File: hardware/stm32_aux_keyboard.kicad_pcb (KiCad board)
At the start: 2 copper layers, 95 x 95 mm, 188 parts, among them J1 I2C_HEADER,2.54, J2 WS2812_HEADER, J3 BUZZER_HEADER, J4 ROT_ENC_HEADER, J5 SWD_SWD, J6 SWD_SWD, J7 ROT_ENC_HEADER, J8 I2C_HEADER,2.54, Q1 SS9013_J3, SW1 USR_BTN_1, SW10 KEY22, SW11 KEY23, SW12 KEY31, SW13 KEY32, SW14 KEY33, SW18 ROT1, SW19 SW_RESET,2_leg,SMD, SW2 USR_BTN_2, SW3 USR_BTN_3, SW5 ROT2, SW6 KEY11, SW7 KEY12, SW8 KEY13, SW9 KEY21, U1 SSD1306-OLED-I2C, U10 STM32F103C8T6, U2 AMS1117-3.3, U3 74AHCT1G125, U4 USB, U5 USBLC6-2SC6_SOT23-6, U6 STM32F103C8T6_rect, U7 SWD, U8 AMS1117-3.3, U9 USBLC6-2SC6_SOT23-6, Y1 O_8M, Y2 O8M, Y3 O32.768K

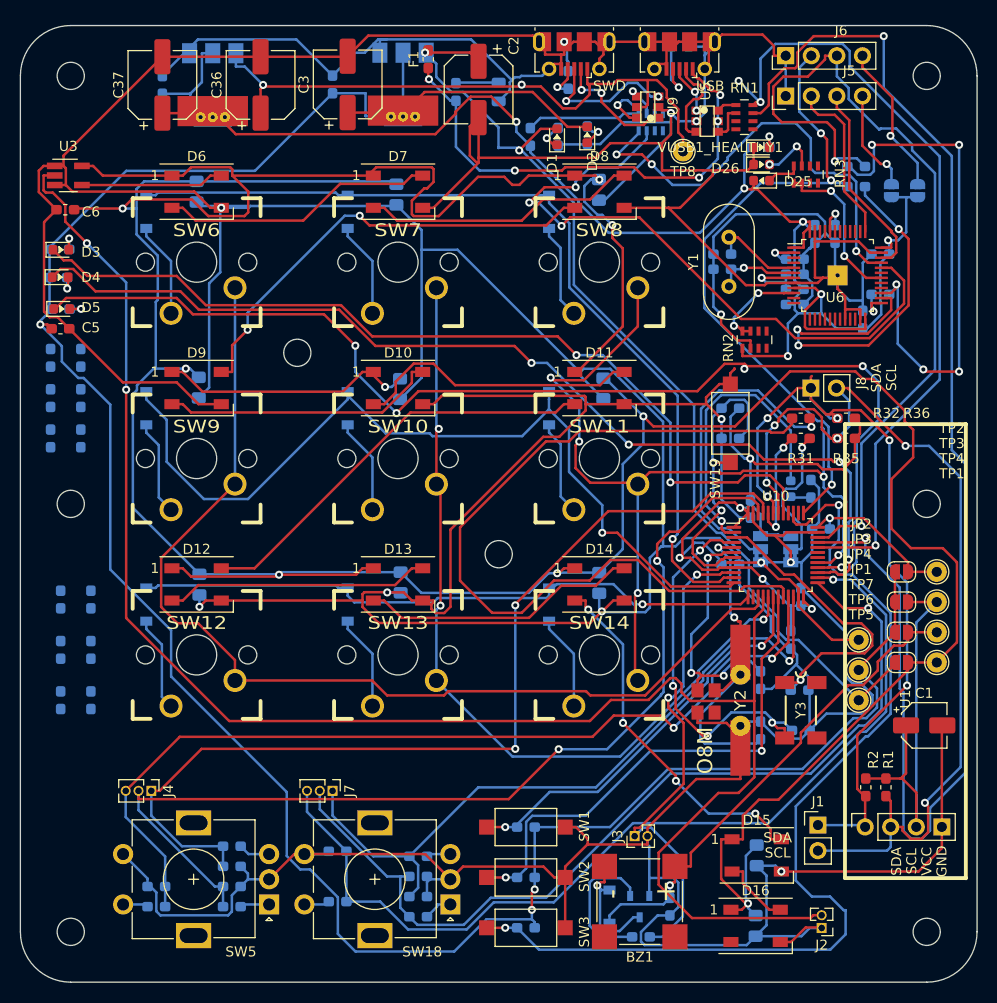
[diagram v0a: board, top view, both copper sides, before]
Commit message: update for autoroute complete,
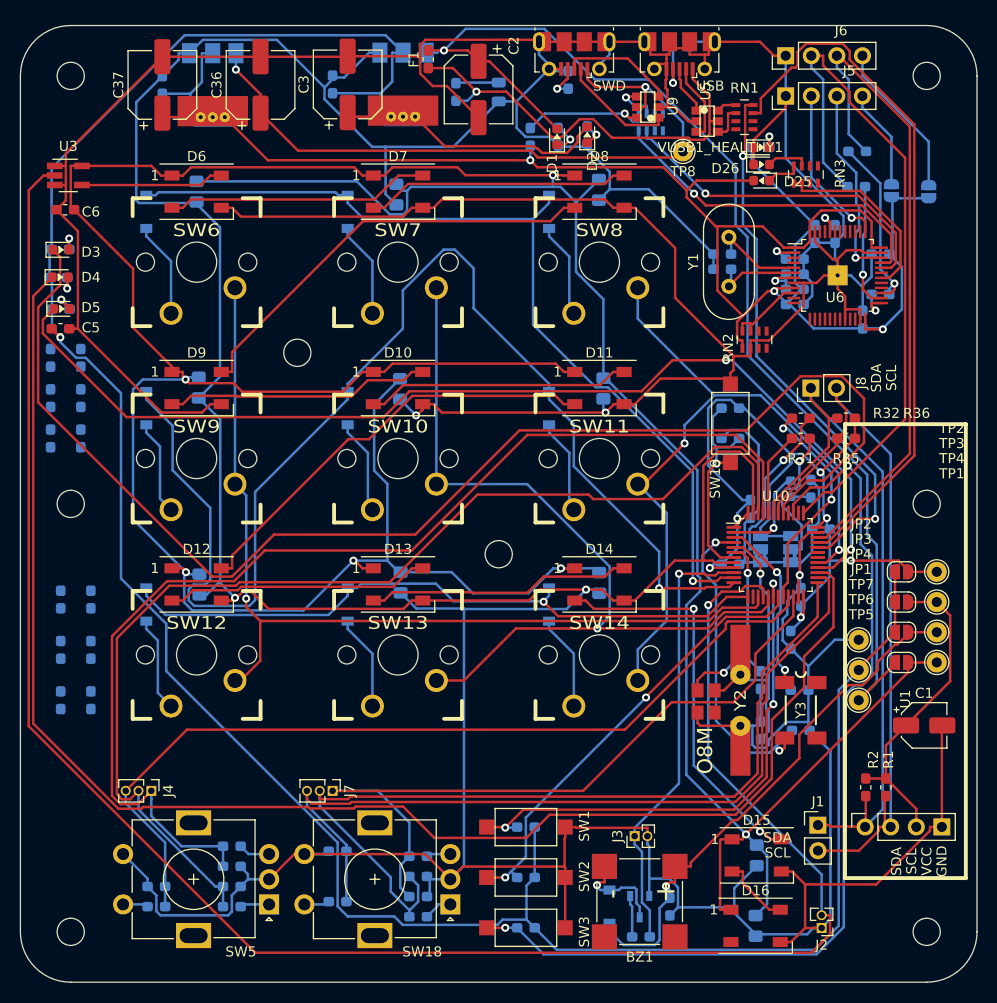
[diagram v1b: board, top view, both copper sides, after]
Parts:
- moved R23 1.50 mm to (103.1, 32.5)
- moved JP6 1.10 mm to (110.2, 36.5)
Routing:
- net GND: track 963.2 -> 885.7 mm, vias 12 -> 5
- net /stm32_core/USB_P: track 141.7 -> 70.4 mm, vias 2 -> 0
- net /stm32_core/BOOT1: track 81.2 -> 22.3 mm, vias 0 -> 2
- net /status_display/USR_LED_2: track 101.2 -> 150.1 mm, vias 4 -> 0
- net /status_display/USR_LED_1: track 88.8 -> 130.5 mm, vias 2 -> 0
- net /keyboard_key/ROW2: track 86.6 -> 125.4 mm
- net /stm32_swd/T_JTMS: track 53.4 -> 18.4 mm, vias 5 -> 1
- net /stm32_swd/USB_N: track 65.4 -> 34.0 mm, vias 3 -> 1
- net /stm32_swd/T_JTCK: track 40.4 -> 12.5 mm, vias 3 -> 1
- net /stm32_core/USB_N: track 79.5 -> 54.3 mm, vias 3 -> 2
- net /oled/SCL: track 94.7 -> 72.9 mm, vias 5 -> 0
- net VCC: track 409.2 -> 387.6 mm, vias 9 -> 6
- net /WS2812/WS2812_IN: track 170.4 -> 191.4 mm, vias 2 -> 1
- net /stm32_core/PC13: track 29.3 -> 9.72 mm
- net +3V3: track 249.7 -> 269.1 mm, vias 3 -> 1
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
